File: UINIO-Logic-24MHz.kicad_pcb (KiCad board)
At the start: 2 copper layers, 48.8 x 25.5 mm, 51 parts, among them J1 Conn_01x10_Pin, U1 AT24CS64-XHM, U2 74HC245C, U3 ME6211C33M5G-N, U4 CY7C68013A-56LTX, Y1 24MHz

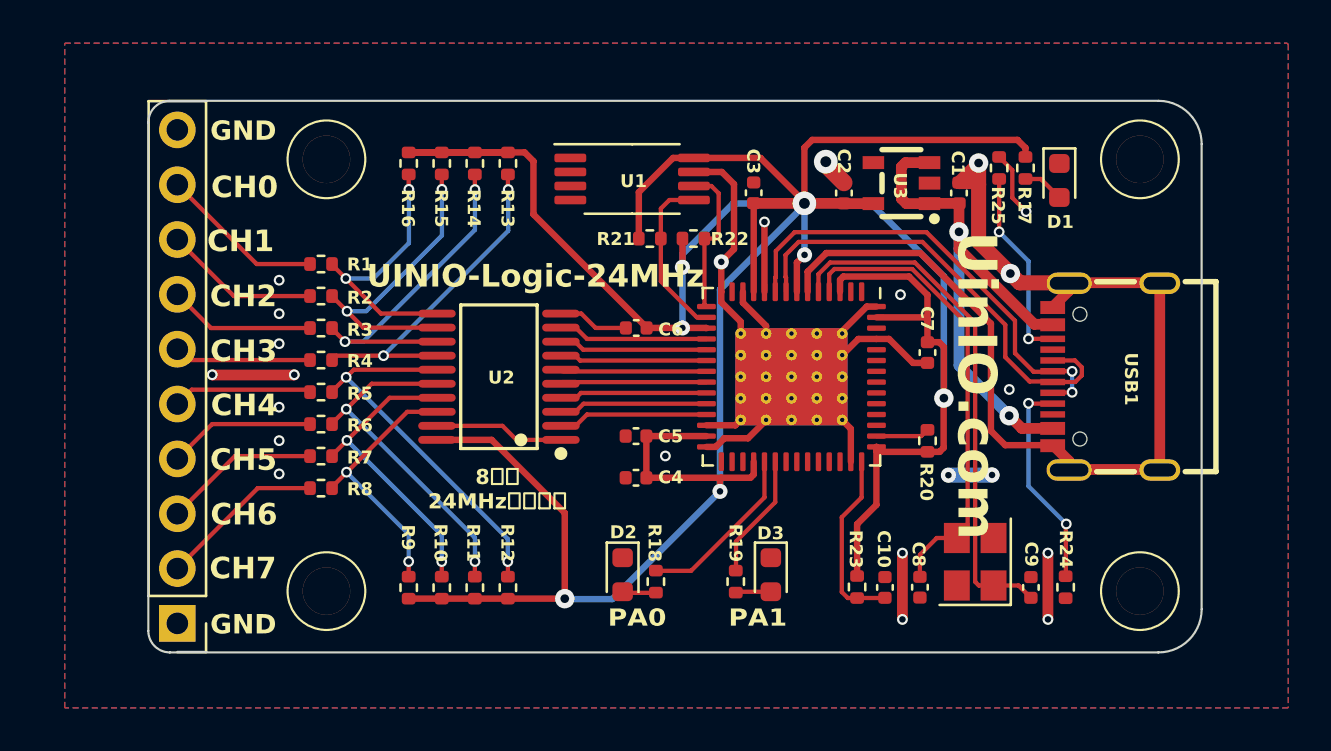
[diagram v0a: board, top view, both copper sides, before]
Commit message: Release UINIO-Logic-24MHz version 3.1.0.
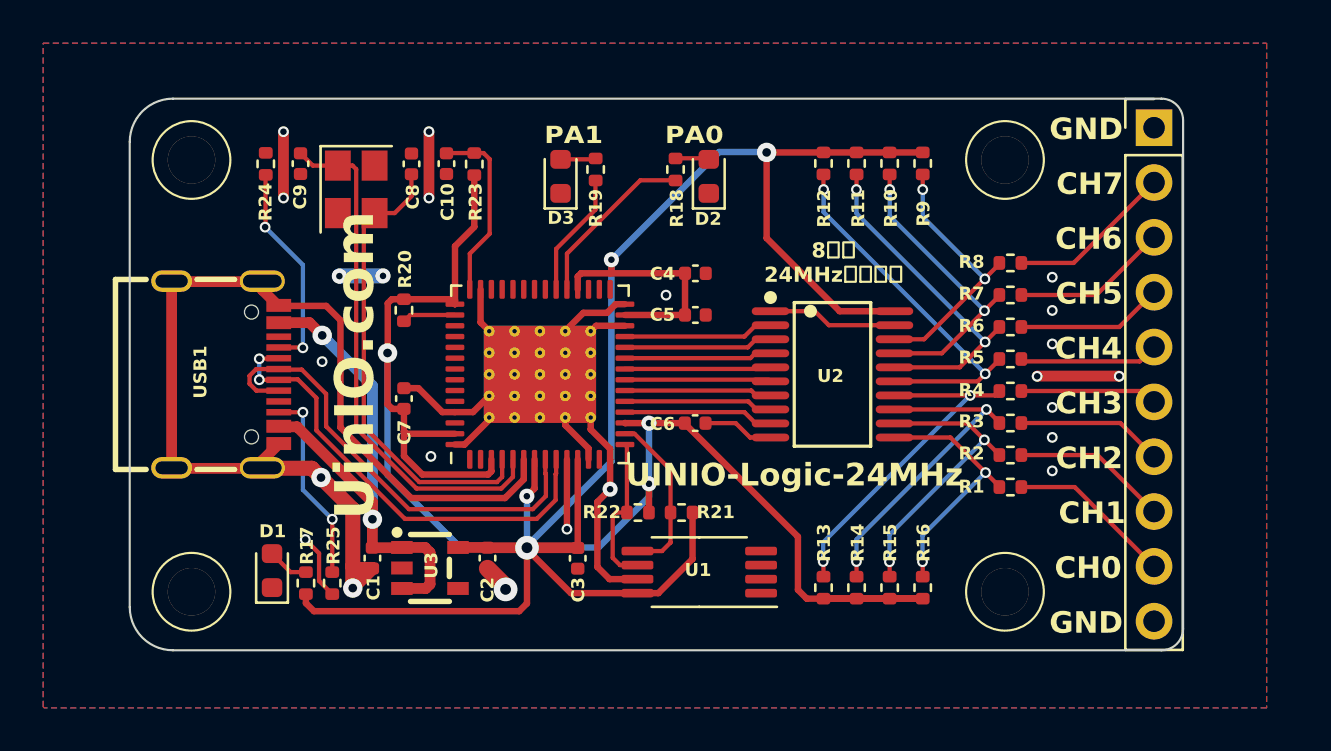
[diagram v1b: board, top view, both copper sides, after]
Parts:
- moved J1 50.7 mm to (174.1, 94.2), turned to 0 degrees
- moved HOLE3 48.3 mm to (129.5, 115.6), turned to 180 degrees
- moved HOLE4 48.3 mm to (129.5, 95.6), turned to 180 degrees
- moved R24 41.9 mm to (132.9, 95.8), turned to 90 degrees
- moved USB1 40.8 mm to (131.0, 105.6), turned to -90 degrees
- moved D1 40.7 mm to (133.2, 114.7), turned to 90 degrees
- moved C9 39.1 mm to (134.5, 95.8), turned to 90 degrees
- moved R17 38.5 mm to (134.8, 115.2), turned to -90 degrees
- moved HOLE1 37.3 mm to (167.2, 115.6), turned to 180 degrees
- moved HOLE2 37.2 mm to (167.2, 95.6), turned to 180 degrees
- moved R25 36.4 mm to (136.0, 115.2), turned to -90 degrees
- moved R8 33.6 mm to (167.4, 100.4), turned to 0 degrees
- moved R1 33.6 mm to (167.4, 110.8), turned to 0 degrees
- moved Y1 33.5 mm to (137.1, 97.0), turned to -90 degrees
- moved R7 32.8 mm to (167.4, 101.9), turned to 0 degrees
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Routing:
- net /INPUT8: track 12.6 -> 11.8 mm
- net /INPUT7: track 14.1 -> 13.6 mm
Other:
- outline, holes or cut-outs redrawn
